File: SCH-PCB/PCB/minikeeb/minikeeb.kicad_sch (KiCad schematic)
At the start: 91 parts, among them J1 OLED, SW1 SW_PUSH-Lily58-cache, SW10 SW_PUSH-Lily58-cache, SW11 SW_PUSH-Lily58-cache, SW12 SW_PUSH-Lily58-cache, SW13 SW_PUSH-Lily58-cache, SW14 SW_PUSH-Lily58-cache, SW15 SW_PUSH-Lily58-cache, SW16 SW_PUSH-Lily58-cache, SW17 SW_PUSH-Lily58-cache, SW18 SW_PUSH-Lily58-cache, SW19 SW_PUSH-Lily58-cache, SW2 SW_PUSH-Lily58-cache, SW20 Rotary_Encoder_Switch-Device, SW3 SW_PUSH-Lily58-cache, SW4 SW_PUSH-Lily58-cache, SW5 SW_PUSH-Lily58-cache, SW6 SW_PUSH-Lily58-cache, SW7 SW_PUSH-Lily58-cache, SW8 SW_PUSH-Lily58-cache, SW9 SW_PUSH-Lily58-cache, U1 ProMicro_2-Lily58-cache, U2 TRRS

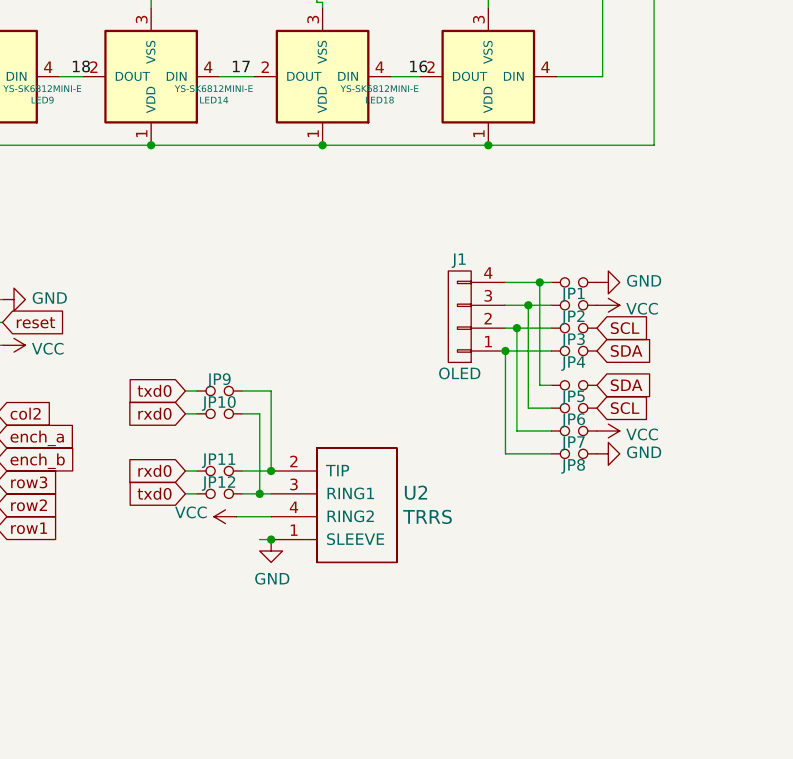
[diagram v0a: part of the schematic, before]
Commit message: FEAT: update pcb
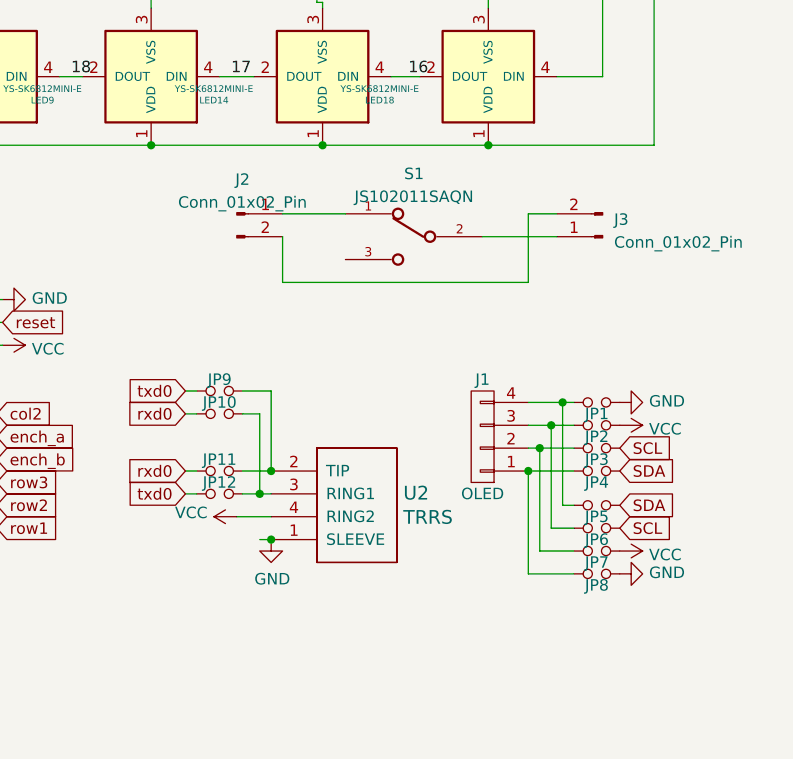
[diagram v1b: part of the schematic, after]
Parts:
- added J2, J3: Conn_01x02_Pin, Connector_JST:JST_EH_B2B-EH-A_1x02_P2.50mm_Vertical, symbol Connector:Conn_01x02_Pin
- added S1: JS102011SAQN, other:SW_JS102011SAQN, symbol other:JS102011SAQN
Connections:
- new net: J3.1 (Pin_1), S1.2
- new net: J2.2 (Pin_2), J3.2 (Pin_2)
- new net: J2.1 (Pin_1), S1.1
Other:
- moved on the sheet: J1, JP1, JP2, JP3, JP4, JP5, JP6, JP7, JP8
